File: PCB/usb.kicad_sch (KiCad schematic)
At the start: 52 parts, among them J2 Conn_ARM_SWD_TagConnect_TC2030, J4 TYPE-C-31-M-12, U10 FT2232HQ, U3 TPD2EUSB30, U4 TPD2EUSB30, U6 TPD2EUSB30, U8 TPS62132, U9 M93C56-WMN6TP, Y2 12MHz

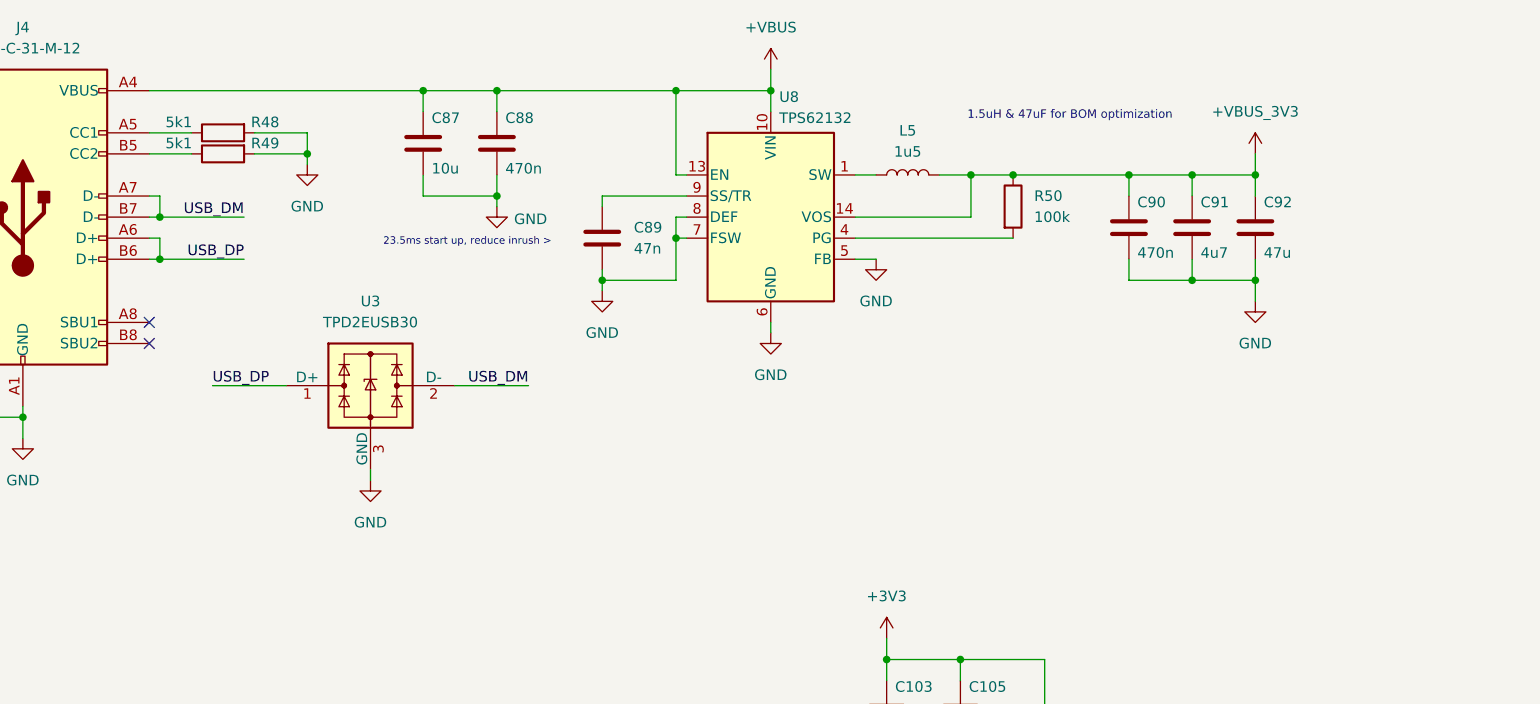
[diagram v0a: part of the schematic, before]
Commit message: cleaning up USB-C, switching some of the decoupling and assigning a bunch of footprints
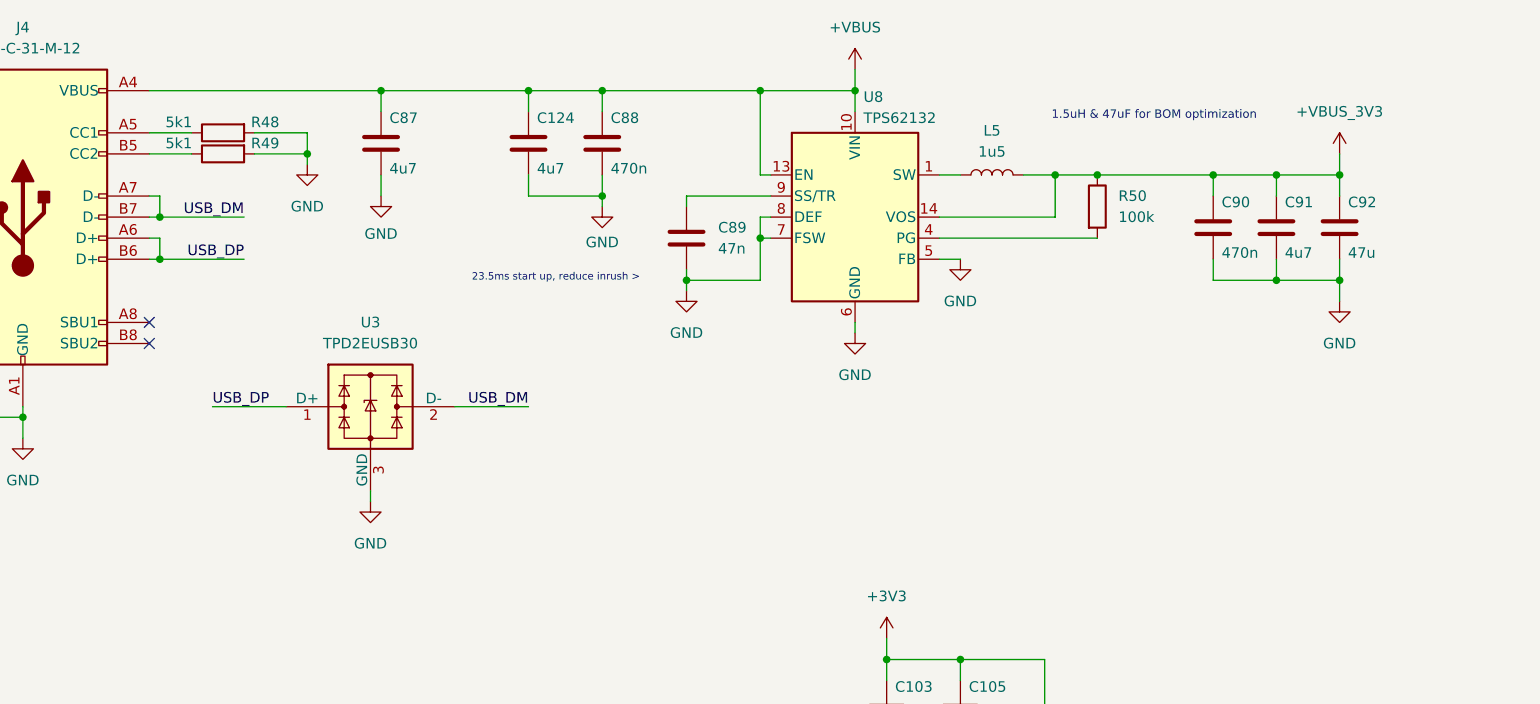
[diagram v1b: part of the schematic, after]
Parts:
- added C124: 4u7, symbol Device:C
- C87: value 10u -> 4u7
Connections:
- net +VBUS: now also C124.1
- net GND: now also C124.2
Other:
- moved on the sheet: C87, C88, C89, C90, C91, C92, L5, R50, U3, U8
